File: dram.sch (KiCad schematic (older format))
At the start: 2 parts

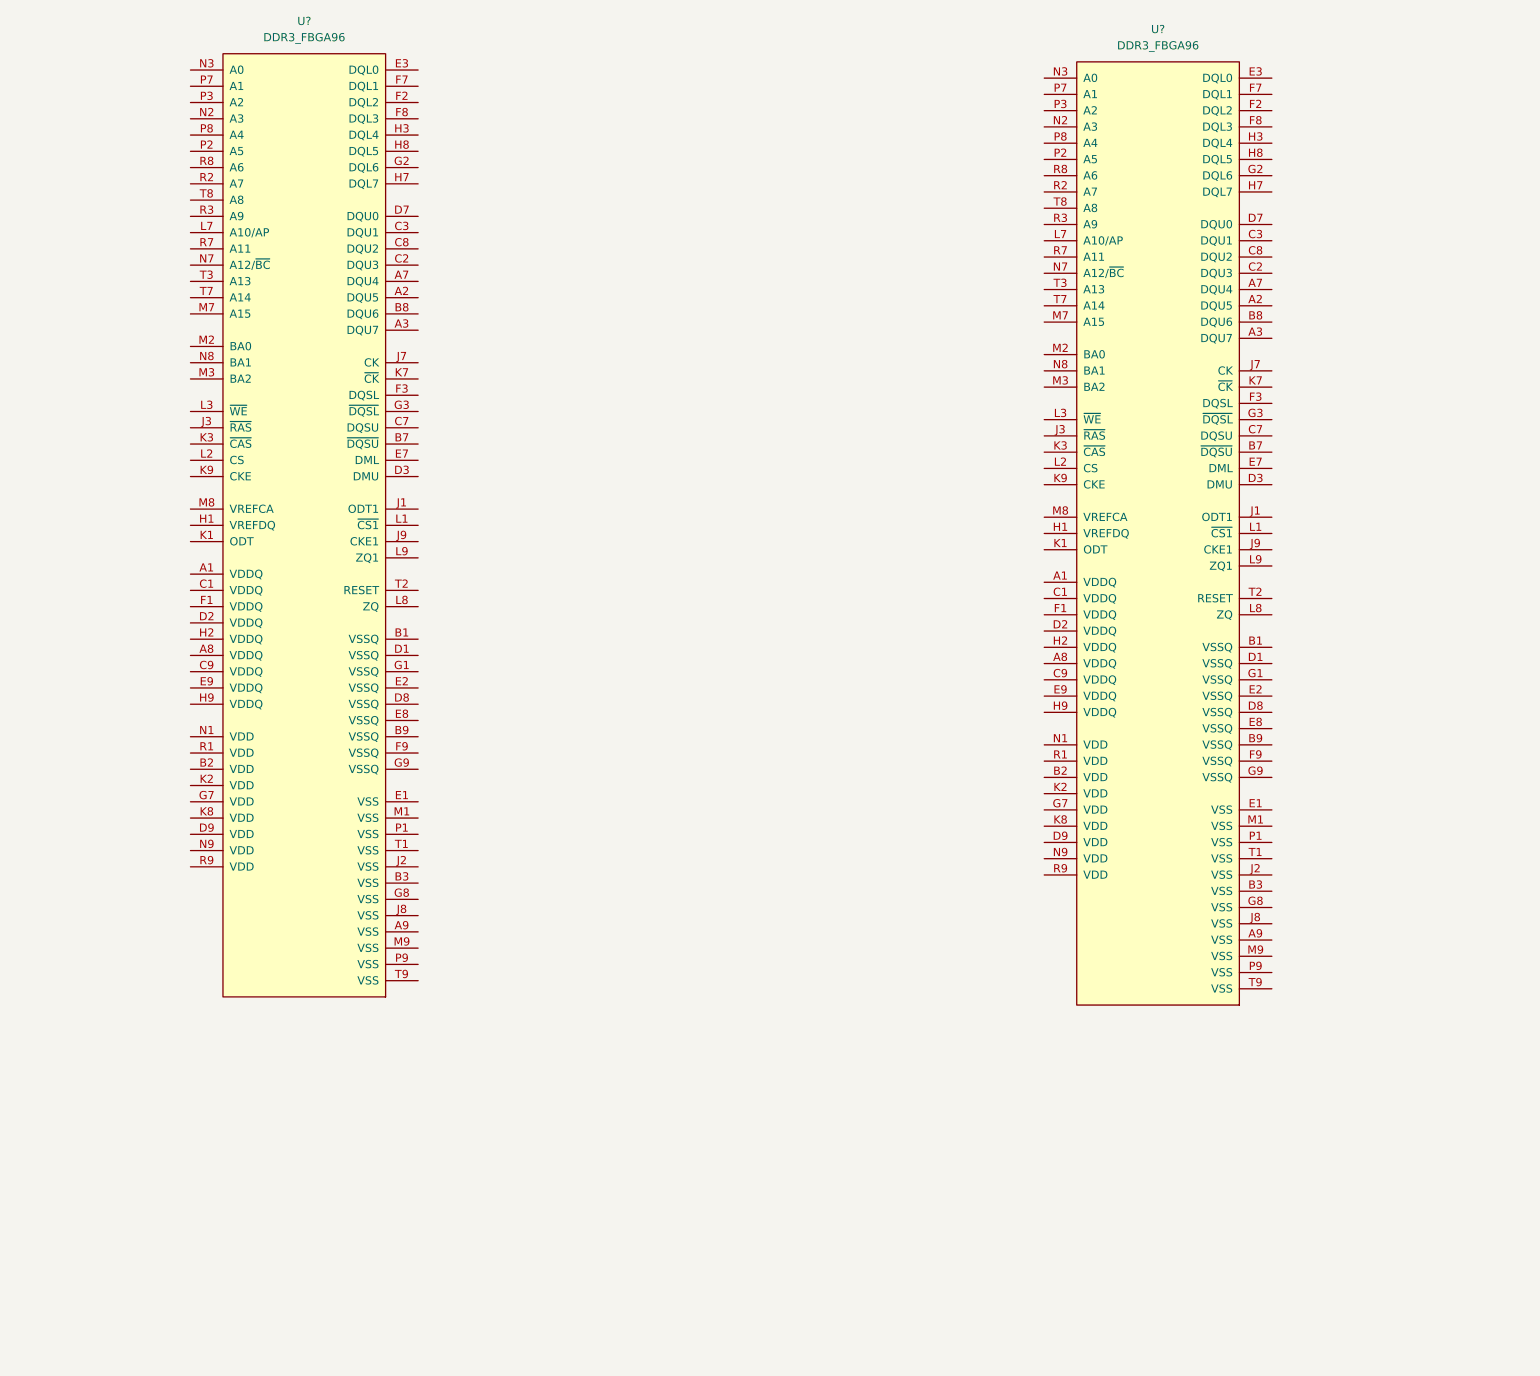
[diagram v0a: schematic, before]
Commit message: update dram,
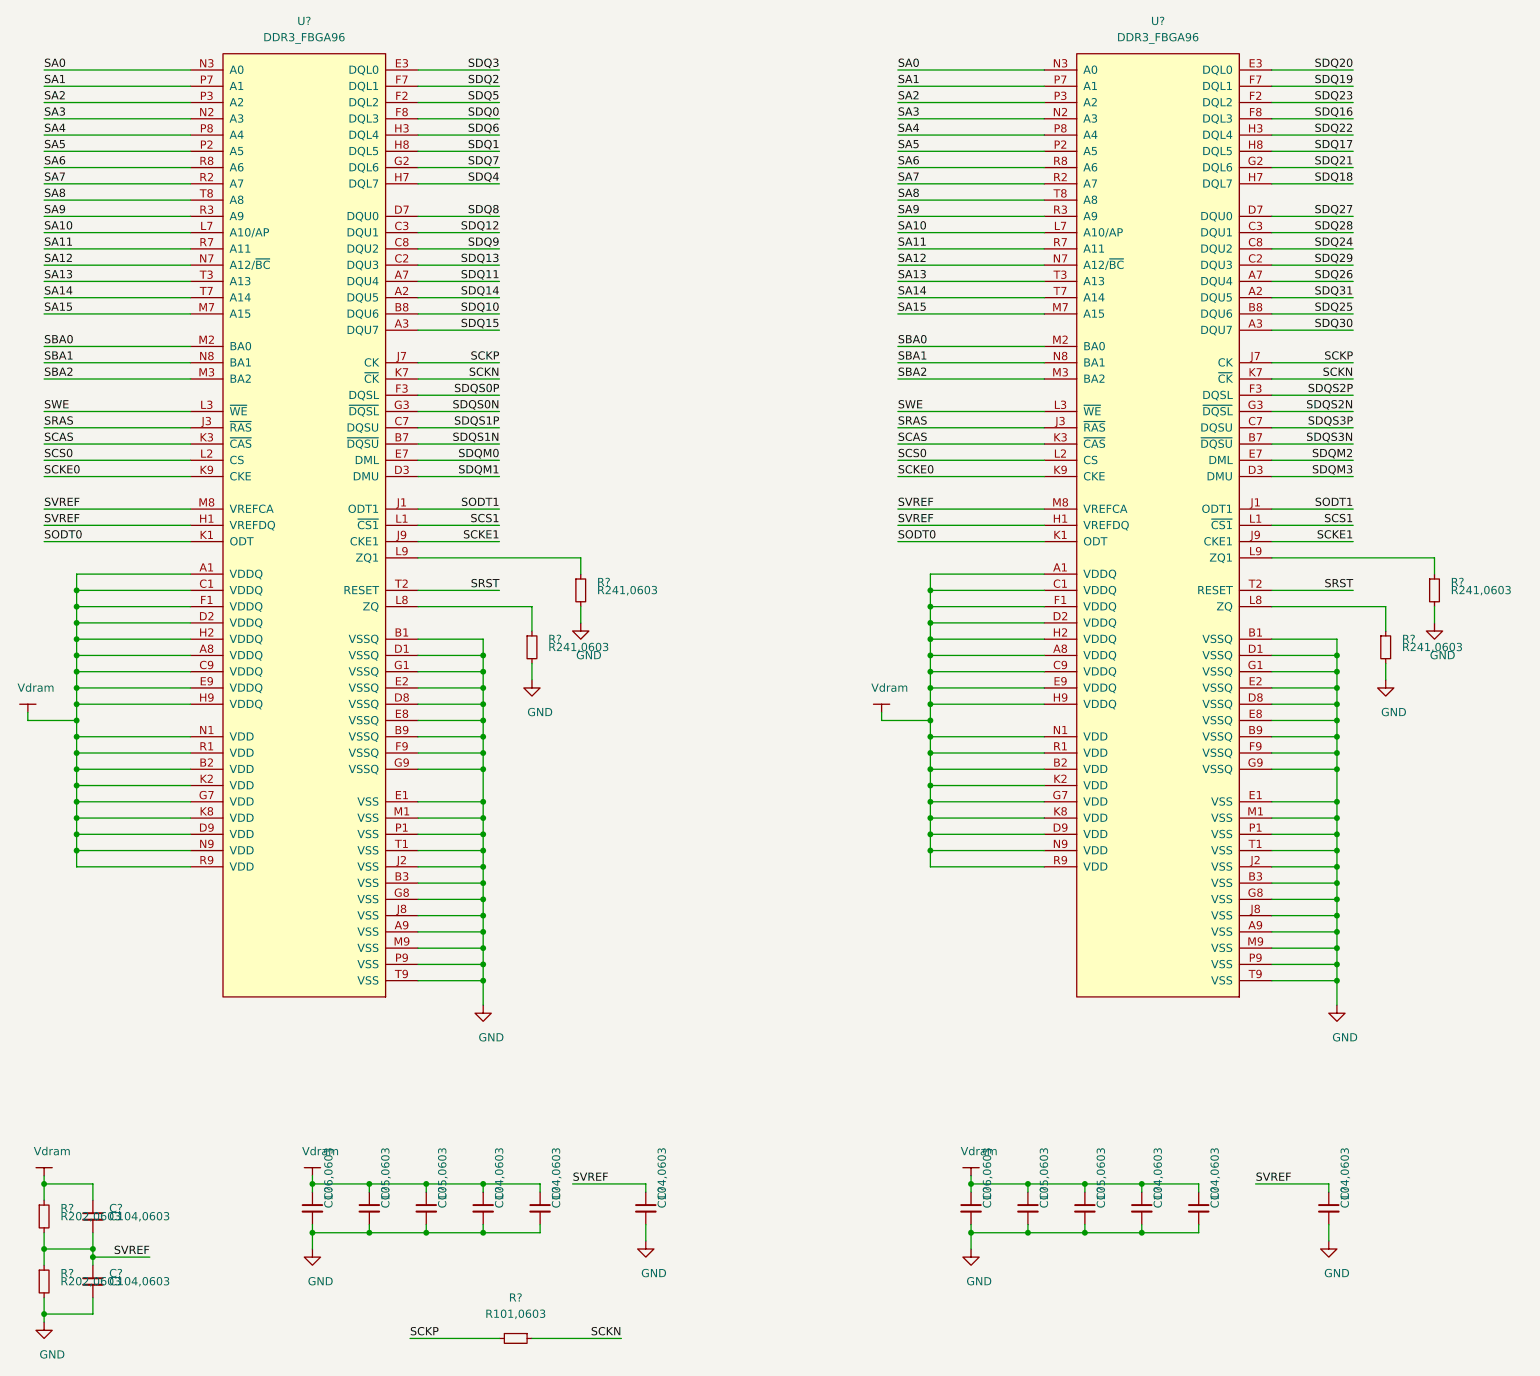
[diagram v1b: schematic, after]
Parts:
- added C? (x8): C104,0603, Capacitor_SMD:C_0603_1608Metric_Pad1.05x0.95mm_HandSolder, symbol taobao-c:C104,0603
- added C? (x2): C106,0603, Capacitor_SMD:C_0603_1608Metric_Pad1.05x0.95mm_HandSolder, symbol taobao-c:C106,0603
- added C? (x4): C105,0603, Capacitor_SMD:C_0603_1608Metric_Pad1.05x0.95mm_HandSolder, symbol taobao-c:C105,0603
- added R? (x4): R241,0603, Resistor_SMD:R_0603_1608Metric_Pad1.05x0.95mm_HandSolder, symbol taobao-r:R241,0603
- added R? (x2): R202,0603, Resistor_SMD:R_0603_1608Metric_Pad1.05x0.95mm_HandSolder, symbol taobao-r:R202,0603
- added R?: R101,0603, Resistor_SMD:R_0603_1608Metric_Pad1.05x0.95mm_HandSolder, symbol taobao-r:R101,0603
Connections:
- net Vdram: now reaches U?.A1 (VDDQ)
- net Vdram: now also U?.A1 (VDDQ), U?.A8 (VDDQ), U?.A8 (VDDQ), U?.B2 (VDD), U?.B2 (VDD), U?.C1 (VDDQ), U?.C1 (VDDQ), U?.C9 (VDDQ), U?.C9 (VDDQ), U?.D2 (VDDQ), U?.D2 (VDDQ), U?.D9 (VDD), U?.D9 (VDD), U?.E9 (VDDQ), U?.E9 (VDDQ), U?.F1 (VDDQ), U?.F1 (VDDQ), U?.G7 (VDD), U?.G7 (VDD), U?.H2 (VDDQ), U?.H2 (VDDQ), U?.H9 (VDDQ), U?.H9 (VDDQ), U?.K2 (VDD), U?.K2 (VDD), U?.K8 (VDD), U?.K8 (VDD), U?.N1 (VDD), U?.N1 (VDD), U?.N9 (VDD), U?.N9 (VDD), U?.R1 (VDD), U?.R1 (VDD), U?.R9 (VDD), U?.R9 (VDD), C?.1, C?.1, C?.1, C?.1, C?.1, C?.1, C?.1, C?.1, C?.1, C?.1, C?.1, R?.1
- net SDQ14: now reaches U?.A2 (DQU5)
- net SDQ15: now reaches U?.A3 (DQU7)
- net SDQ11: now reaches U?.A7 (DQU4)
- net GND: now reaches U?.A9 (VSS)
- net GND: now also U?.A9 (VSS), U?.B1 (VSSQ), U?.B1 (VSSQ), U?.B3 (VSS), U?.B3 (VSS), U?.B9 (VSSQ), U?.B9 (VSSQ), U?.D1 (VSSQ), U?.D1 (VSSQ), U?.D8 (VSSQ), U?.D8 (VSSQ), U?.E1 (VSS), U?.E1 (VSS), U?.E2 (VSSQ), U?.E2 (VSSQ), U?.E8 (VSSQ), U?.E8 (VSSQ), U?.F9 (VSSQ), U?.F9 (VSSQ), U?.G1 (VSSQ), U?.G1 (VSSQ), U?.G8 (VSS), U?.G8 (VSS), U?.G9 (VSSQ), U?.G9 (VSSQ), U?.J2 (VSS), U?.J2 (VSS), U?.J8 (VSS), U?.J8 (VSS), U?.M1 (VSS), U?.M1 (VSS), U?.M9 (VSS), U?.M9 (VSS), U?.P1 (VSS), U?.P1 (VSS), U?.P9 (VSS), U?.P9 (VSS), U?.T1 (VSS), U?.T1 (VSS), U?.T9 (VSS), U?.T9 (VSS), C?.2, C?.2, C?.2, C?.2, C?.2, C?.2, C?.2, C?.2, C?.2, C?.2, C?.2, C?.2, C?.2, R?.2, R?.2, R?.2, R?.2, R?.2
- net SDQS1N: now reaches U?.B7 (~DQSU~)
- net SDQ10: now reaches U?.B8 (DQU6)
- net SDQ13: now reaches U?.C2 (DQU3)
- net SDQ12: now reaches U?.C3 (DQU1)
- net SDQS1P: now reaches U?.C7 (DQSU)
- net SDQ9: now reaches U?.C8 (DQU2)
- net SDQM1: now reaches U?.D3 (DMU)
- net SDQ8: now reaches U?.D7 (DQU0)
- net SDQ3: now reaches U?.E3 (DQL0)
- net SDQM0: now reaches U?.E7 (DML)
- net SDQ5: now reaches U?.F2 (DQL2)
- net SDQS0P: now reaches U?.F3 (DQSL)
- net SDQ2: now reaches U?.F7 (DQL1)
- net SDQ0: now reaches U?.F8 (DQL3)
- net SDQ7: now reaches U?.G2 (DQL6)
- net SDQS0N: now reaches U?.G3 (~DQSL~)
- net SVREF: now reaches U?.H1 (VREFDQ)
- net SVREF: now also U?.H1 (VREFDQ), U?.M8 (VREFCA), U?.M8 (VREFCA), C?.1, C?.1, C?.1, C?.2, R?.1, R?.2
- net SDQ6: now reaches U?.H3 (DQL4)
- net SDQ4: now reaches U?.H7 (DQL7)
- net SDQ1: now reaches U?.H8 (DQL5)
- net SODT1: now reaches U?.J1 (ODT1)
- net SODT1: now also U?.J1 (ODT1)
- net SRAS: now reaches U?.J3 (~RAS~)
- net SRAS: now also U?.J3 (~RAS~)
- net SCKP: now reaches U?.J7 (CK)
- net SCKP: now also U?.J7 (CK), R?.2
- net SCKE1: now reaches U?.J9 (CKE1)
- net SCKE1: now also U?.J9 (CKE1)
- net SODT0: now reaches U?.K1 (ODT)
- net SODT0: now also U?.K1 (ODT)
- net SCAS: now reaches U?.K3 (~CAS~)
- net SCAS: now also U?.K3 (~CAS~)
- net SCKN: now reaches U?.K7 (~CK~)
- net SCKN: now also U?.K7 (~CK~), R?.1
- net SCKE0: now reaches U?.K9 (CKE)
- net SCKE0: now also U?.K9 (CKE)
- net SCS1: now reaches U?.L1 (~CS1~)
- net SCS1: now also U?.L1 (~CS1~)
- net SCS0: now reaches U?.L2 (CS)
- net SCS0: now also U?.L2 (CS)
- net SWE: now reaches U?.L3 (~WE~)
- net SWE: now also U?.L3 (~WE~)
- net SA10: now reaches U?.L7 (A10/AP)
- net SA10: now also U?.L7 (A10/AP)
- net at U?.L8 (ZQ): now also R?.1 (x2)
- net at U?.L9 (ZQ1): now also R?.1 (x2)
- net SBA0: now reaches U?.M2 (BA0)
- net SBA0: now also U?.M2 (BA0)
- net SBA2: now reaches U?.M3 (BA2)
- net SBA2: now also U?.M3 (BA2)
- net SA15: now reaches U?.M7 (A15)
- net SA15: now also U?.M7 (A15)
- net SA3: now reaches U?.N2 (A3)
- net SA3: now also U?.N2 (A3)
- net SA0: now reaches U?.N3 (A0)
- net SA0: now also U?.N3 (A0)
- net SA12: now reaches U?.N7 (A12/~BC~)
- net SA12: now also U?.N7 (A12/~BC~)
- net SBA1: now reaches U?.N8 (BA1)
- net SBA1: now also U?.N8 (BA1)
- net SA5: now reaches U?.P2 (A5)
- net SA5: now also U?.P2 (A5)
- net SA2: now reaches U?.P3 (A2)
- net SA2: now also U?.P3 (A2)
- net SA1: now reaches U?.P7 (A1)
- net SA1: now also U?.P7 (A1)
- net SA4: now reaches U?.P8 (A4)
- net SA4: now also U?.P8 (A4)
- net SA7: now reaches U?.R2 (A7)
- net SA7: now also U?.R2 (A7)
- net SA9: now reaches U?.R3 (A9)
- net SA9: now also U?.R3 (A9)
- net SA11: now reaches U?.R7 (A11)
- net SA11: now also U?.R7 (A11)
- net SA6: now reaches U?.R8 (A6)
- net SA6: now also U?.R8 (A6)
- net SRST: now reaches U?.T2 (RESET)
- net SRST: now also U?.T2 (RESET)
- net SA13: now reaches U?.T3 (A13)
- net SA13: now also U?.T3 (A13)
- net SA14: now reaches U?.T7 (A14)
- net SA14: now also U?.T7 (A14)
- net SA8: now reaches U?.T8 (A8)
- net SA8: now also U?.T8 (A8)
- net SDQ31: now reaches U?.A2 (DQU5)
- net SDQ30: now reaches U?.A3 (DQU7)
- net SDQ26: now reaches U?.A7 (DQU4)
- net SDQS3N: now reaches U?.B7 (~DQSU~)
- net SDQ25: now reaches U?.B8 (DQU6)
- net SDQ29: now reaches U?.C2 (DQU3)
- net SDQ28: now reaches U?.C3 (DQU1)
- net SDQS3P: now reaches U?.C7 (DQSU)
- net SDQ24: now reaches U?.C8 (DQU2)
- net SDQM3: now reaches U?.D3 (DMU)
- net SDQ27: now reaches U?.D7 (DQU0)
- net SDQ20: now reaches U?.E3 (DQL0)
- net SDQM2: now reaches U?.E7 (DML)
- net SDQ23: now reaches U?.F2 (DQL2)
- net SDQS2P: now reaches U?.F3 (DQSL)
- net SDQ19: now reaches U?.F7 (DQL1)
- net SDQ16: now reaches U?.F8 (DQL3)
- net SDQ21: now reaches U?.G2 (DQL6)
- net SDQS2N: now reaches U?.G3 (~DQSL~)
- net SDQ22: now reaches U?.H3 (DQL4)
- net SDQ18: now reaches U?.H7 (DQL7)
- net SDQ17: now reaches U?.H8 (DQL5)
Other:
- moved on the sheet: U?
